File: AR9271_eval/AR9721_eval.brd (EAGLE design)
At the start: 94 x 80 mm, 125 parts, among them J1 UJ2-MIBH2-4-SMT-TR, J3 HTST-110-01-XX-DV, J7 132134-15, J8 132134-15, U1 U-ATHEROS-AR9271, U2 AT24C04C-XHM-T, U3 LT3080EQPBF, U4 LT3080EQPBF, U5 LT3080EQPBF, U6 LT3080EQPBF, Y1 ECS-400-10-36-CKY-TR

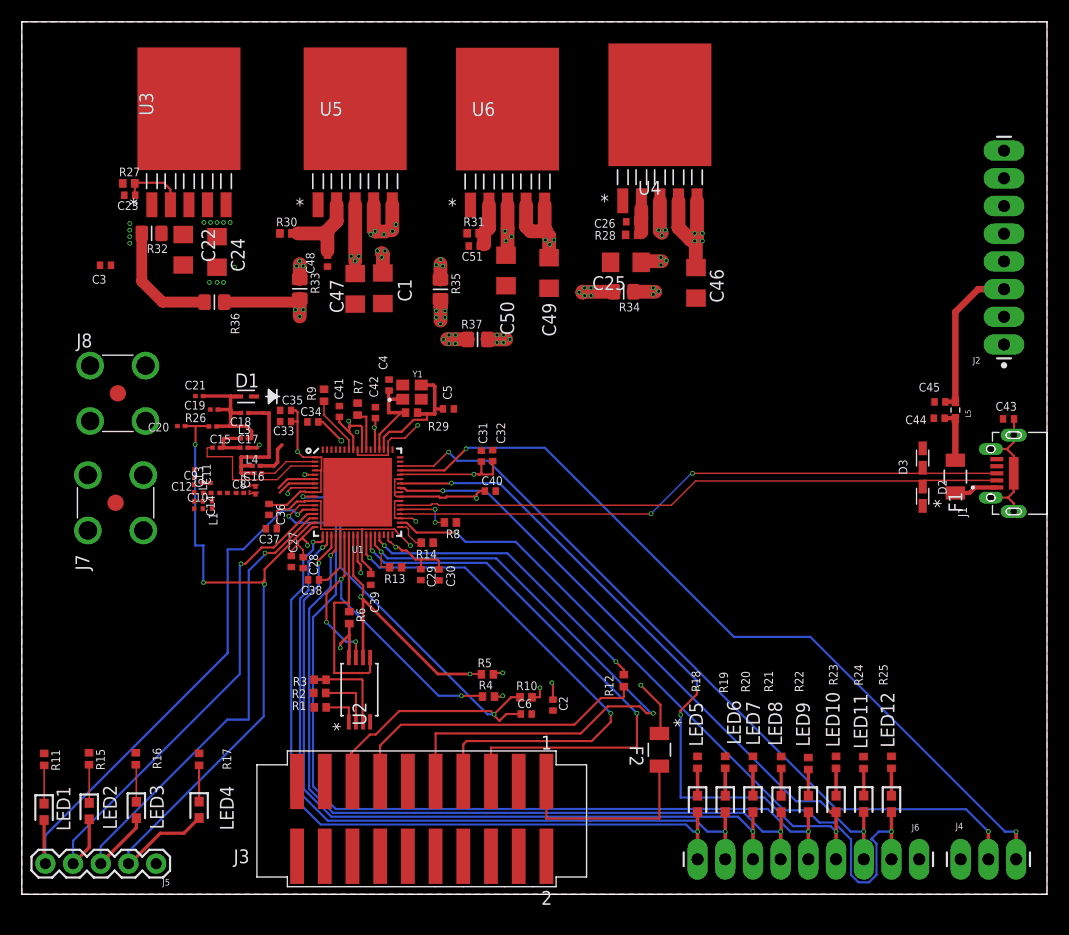
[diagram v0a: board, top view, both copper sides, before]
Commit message: Here's my newest update to the AR9721 board
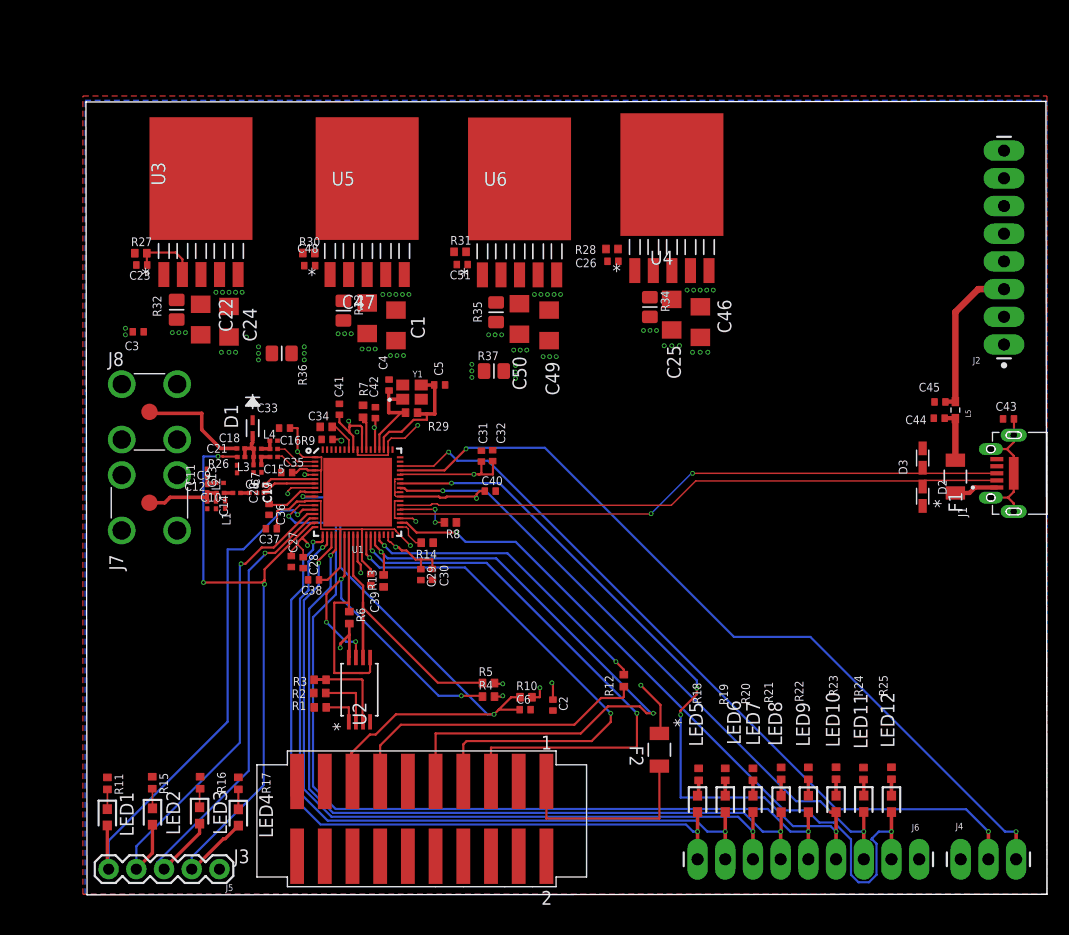
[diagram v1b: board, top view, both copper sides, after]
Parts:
- moved R36 7.76 mm to (23.8, 49.6)
- moved R32 7.37 mm to (14.2, 53.6), turned to 270 degrees
- moved C3 6.80 mm to (10.7, 51.6)
- moved C22 6.60 mm to (16.4, 52.7)
- moved C19 6.52 mm to (21.2, 39.0), turned to 270 degrees
- moved R27 6.49 mm to (10.9, 58.8)
- moved U5 6.49 mm to (31.7, 65.6)
- moved U6 6.49 mm to (45.6, 65.6)
- moved U3 6.49 mm to (16.4, 65.6)
- moved C24 6.49 mm to (19.0, 52.5)
- moved C23 6.49 mm to (11.0, 57.7)
- moved U4 6.49 mm to (59.6, 66.0)
- moved C20 6.46 mm to (19.7, 39.0), turned to 270 degrees
- moved C25 6.38 mm to (59.6, 53.1), turned to 270 degrees
- moved R16 6.30 mm to (16.4, 10.2)
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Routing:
- net LDO_IN: track 51.2 -> 12.1 mm
- net 3V3_D: track 95.8 -> 70.7 mm, vias 17 -> 19
- net N$43: track 14.6 -> 0.00 mm
- net N$47: track 14.2 -> 0.00 mm, vias 6 -> 0
- net N$37: track 13.5 -> 0.00 mm, vias 9 -> 0
- net N$44: track 13.0 -> 0.00 mm, vias 6 -> 0
- net N$4: track 38.6 -> 25.8 mm, vias 2 -> 0
- net 3V3_A: track 64.4 -> 52.1 mm, vias 7 -> 10
- net RCV_IN: track 0.03 -> 10.3 mm
- net N$17: track 12.1 -> 1.80 mm
- net RFIN_P: track 13.8 -> 3.87 mm
- net N$24: track 12.8 -> 4.43 mm
- net XMIT_OUT: track 0.00 -> 7.99 mm
- net SWCOM3: track 69.9 -> 63.1 mm
- net 1V2_A: track 28.0 -> 21.8 mm, vias 12 -> 8
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- added copper zone on layer 15, net 3V3_A
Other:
- board size 94 x 80 mm -> 88.1 x 72.7 mm
